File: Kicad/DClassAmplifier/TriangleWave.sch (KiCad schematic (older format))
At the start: 7 parts, among them U2 MAX4016ESA+

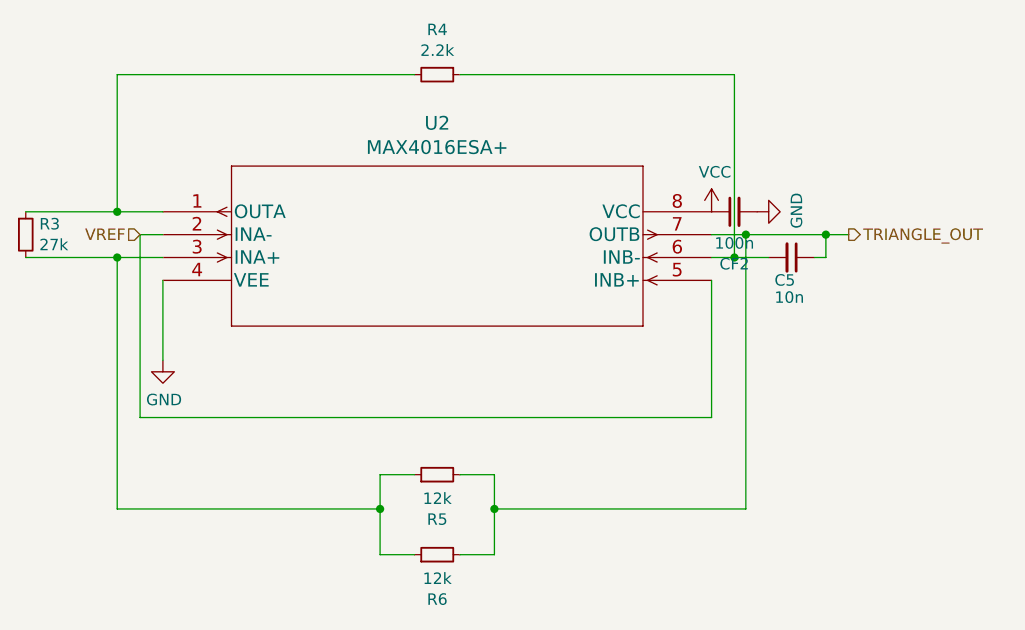
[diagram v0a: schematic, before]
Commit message: Combined Board
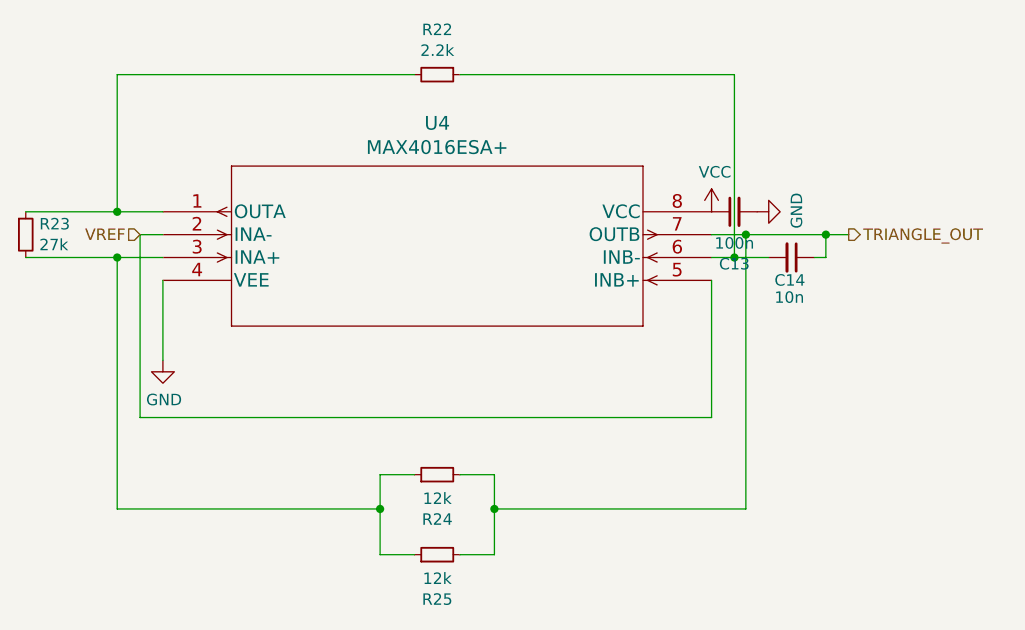
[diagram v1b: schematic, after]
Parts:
- C13: renamed from CF2; footprint Capacitor_SMD:C_0805_2012Metric_Pad1.18x1.45mm_HandSolder -> Capacitor_SMD:C_0603_1608Metric_Pad1.08x0.95mm_HandSolder
- C14: renamed from C5; footprint Capacitor_SMD:C_0201_0603Metric_Pad0.64x0.40mm_HandSolder -> Capacitor_SMD:C_0603_1608Metric_Pad1.08x0.95mm_HandSolder
- renumbered R4 to R22, R3 to R23, R5 to R24, R6 to R25, U2 to U4
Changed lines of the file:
@@
 $EndDescr
 $Comp
-L power:VCC #PWR015
+L power:VCC #PWR039
 U 1 1 610A2484
 P 6500 3450
-F 0 "#PWR015" H 6500 3300 50  0001 C CNN
+F 0 "#PWR039" H 6500 3300 50  0001 C CNN
 F 1 "VCC" H 6515 3623 50  0000 C CNN
 F 2 "" H 6500 3450 50  0001 C CNN
@@
 $EndComp
 $Comp
-L power:GND #PWR014
+L power:GND #PWR041
 U 1 1 610A5C03
 P 4100 4100
-F 0 "#PWR014" H 4100 3850 50  0001 C CNN
+F 0 "#PWR041" H 4100 3850 50  0001 C CNN
 F 1 "GND" H 4105 3927 50  0000 C CNN
 F 2 "" H 4100 4100 50  0001 C CNN
@@
 TRIANGLE_OUT
 $Comp
-L Device:R_Small R4
+L Device:R_Small R22
 U 1 1 610ABFC7
 P 5300 2850
-F 0 "R4" V 5104 2850 50  0000 C CNN
+F 0 "R22" V 5104 2850 50  0000 C CNN
 F 1 "2.2k" V 5195 2850 50  0000 C CNN
 F 2 "Resistor_SMD:R_0603_1608Metric_Pad0.98x0.95mm_HandSolder" H 5300 2850 50  0001 C CNN
@@
 	4100 4100 4100 3750
 $Comp
-L Device:C_Small C5
+L Device:C_Small C14
 U 1 1 610B0597
 P 6850 3650
-F 0 "C5" V 6950 3575 50  0000 L CNN
+F 0 "C14" V 6950 3575 50  0000 L CNN
 F 1 "10n" V 7025 3575 50  0000 L CNN
-F 2 "Capacitor_SMD:C_0201_0603Metric_Pad0.64x0.40mm_HandSolder" H 6850 3650 50  0001 C CNN
+F 2 "Capacitor_SMD:C_0603_1608Metric_Pad1.08x0.95mm_HandSolder" H 6850 3650 50  0001 C CNN
 F 3 "~" H 6850 3650 50  0001 C CNN
 	1    6850 3650
@@
 	7000 3550 7100 3550
 $Comp
-L Device:R_Small R5
+L Device:R_Small R24
 U 1 1 610B770E
 P 5300 4600
-F 0 "R5" V 5104 4600 50  0000 C CNN
+F 0 "R24" V 5104 4600 50  0000 C CNN
 F 1 "12k" V 5195 4600 50  0000 C CNN
 F 2 "Resistor_SMD:R_0603_1608Metric_Pad0.98x0.95mm_HandSolder" H 5300 4600 50  0001 C CNN
@@
 	3900 3450 3500 3450
 $Comp
-L Device:R_Small R3
+L Device:R_Small R23
 U 1 1 610B9D20
 P 3500 3550
-F 0 "R3" H 3559 3596 50  0000 L CNN
+F 0 "R23" H 3559 3596 50  0000 L CNN
 F 1 "27k" H 3559 3505 50  0000 L CNN
 F 2 "Resistor_SMD:R_0603_1608Metric_Pad0.98x0.95mm_HandSolder" H 3500 3550 50  0001 C CNN
@@
 	6600 3650 6750 3650
 $Comp
-L Device:R_Small R6
+L Device:R_Small R25
 U 1 1 6110AB92
 P 5300 4950
-F 0 "R6" V 5104 4950 50  0000 C CNN
+F 0 "R25" V 5104 4950 50  0000 C CNN
 F 1 "12k" V 5195 4950 50  0000 C CNN
 F 2 "Resistor_SMD:R_0603_1608Metric_Pad0.98x0.95mm_HandSolder" H 5300 4950 50  0001 C CNN
@@
 	5050 4750 5050 4950
 $Comp
-L DClassAmplifier-rescue:MAX4016ESA+-MAX4016ESA U2
+L DClassAmplifier-rescue:MAX4016ESA+-MAX4016ESA U4
 U 1 1 610FB9E0
 P 4100 3450
-F 0 "U2" H 5300 3837 60  0000 C CNN
+F 0 "U4" H 5300 3837 60  0000 C CNN
 F 1 "MAX4016ESA+" H 5300 3731 60  0000 C CNN
 F 2 "MAX4016ESA:MAX4016ESA&plus_" H 5300 3690 60  0001 C CNN
@@
 $EndComp
 $Comp
-L Device:C_Small CF?
+L Device:C_Small C?
 U 1 1 611DAEFE
 P 6600 3450
-AR Path="/610C616D/611DAEFE" Ref="CF?"  Part="1"
-AR Path="/611D4178/611DAEFE" Ref="CF?"  Part="1"
-AR Path="/6109BB03/611DAEFE" Ref="CF2"  Part="1"
-F 0 "CF2" V 6371 3450 50  0000 C CNN
+AR Path="/610C616D/611DAEFE" Ref="C?"  Part="1"
+AR Path="/611D4178/611DAEFE" Ref="C?"  Part="1"
+AR Path="/6109BB03/611DAEFE" Ref="C13"  Part="1"
+F 0 "C13" V 6371 3450 50  0000 C CNN
 F 1 "100n" V 6462 3450 50  0000 C CNN
-F 2 "Capacitor_SMD:C_0805_2012Metric_Pad1.18x1.45mm_HandSolder" H 6600 3450 50  0001 C CNN
+F 2 "Capacitor_SMD:C_0603_1608Metric_Pad1.08x0.95mm_HandSolder" H 6600 3450 50  0001 C CNN
 F 3 "~" H 6600 3450 50  0001 C CNN
 	1    6600 3450
@@
 $EndComp
 $Comp
-L power:GND #PWR?
+L power:GND #PWR040
 U 1 1 611DAF04
 P 6700 3450
-F 0 "#PWR?" H 6700 3200 50  0001 C CNN
+F 0 "#PWR040" H 6700 3200 50  0001 C CNN
 F 1 "GND" H 6705 3277 50  0000 C CNN
 F 2 "" H 6700 3450 50  0001 C CNN
